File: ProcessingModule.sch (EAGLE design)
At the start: 32 parts, among them IC1 INA128U, IC2 LM358MX, IC3 MCP606-I_SN

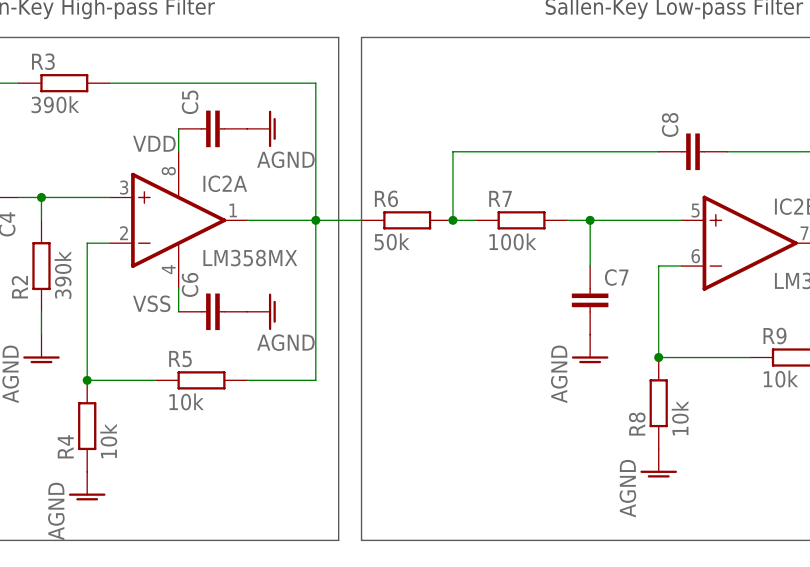
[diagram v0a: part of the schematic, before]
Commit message: Control module first version and Processing module final design
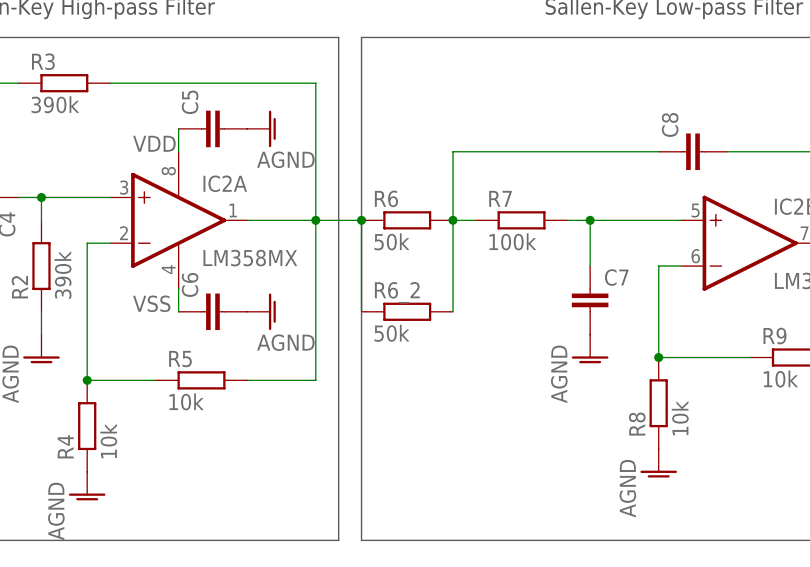
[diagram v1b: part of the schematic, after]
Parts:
- added R6_2: 50k, rcl:R-EU_R0805
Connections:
- net N$11: now also R6_2.2
- net N$4: now also R6_2.1
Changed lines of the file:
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@@
 <part name="R12" library="rcl" library_urn="urn:adsk.eagle:library:334" deviceset="R-EU_" device="R0805" package3d_urn="urn:adsk.eagle:package:23553/2" value="10k"/>
 <part name="R13" library="rcl" library_urn="urn:adsk.eagle:library:334" deviceset="R-EU_" device="R0805" package3d_urn="urn:adsk.eagle:package:23553/2" value="180k"/>
+<part name="R6_2" library="rcl" library_urn="urn:adsk.eagle:library:334" deviceset="R-EU_" device="R0805" package3d_urn="urn:adsk.eagle:package:23553/2" value="50k"/>
 </parts>
 <sheets>
@@
 <instance part="R12" gate="G$1" x="25.4" y="17.78" rot="R90"/>
 <instance part="R13" gate="G$1" x="38.1" y="48.26"/>
+<instance part="R6_2" gate="G$1" x="134.62" y="88.9"/>
 </instances>
 <busses>
@@
 <pinref part="R6" gate="G$1" pin="1"/>
 <wire x1="129.54" y1="99.06" x2="124.46" y2="99.06" width="0.1524" layer="91"/>
+<pinref part="R6_2" gate="G$1" pin="1"/>
+<wire x1="129.54" y1="88.9" x2="129.54" y2="99.06" width="0.1524" layer="91"/>
+<junction x="129.54" y="99.06"/>
 </segment>
 </net>
@@
 <wire x1="139.7" y1="99.06" x2="139.7" y2="106.68" width="0.1524" layer="91"/>
 <junction x="139.7" y="99.06"/>
-</segment>
-</net>
+<pinref part="R6_2" gate="G$1" pin="2"/>
+<wire x1="139.7" y1="88.9" x2="139.7" y2="99.06" width="0.1524" layer="91"/>
+</segment>
+</net>
